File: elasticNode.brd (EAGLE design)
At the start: 58.2 x 52.5 mm, 135 parts, among them J1 FEMALE_HEADER_2X1, J2 JUMPER, J3 JUMPER, J5 FEMALE_HEADER_10X2, J6 USB_CONNMICRO_SMT, J7 USB_CONNMICRO_SMT, M1 SISS23DN, M2 SISS23DN, M3 SISS23DN, M4 SISS23DN, U1 AT90USB128, U10 LTC3419DFN, U11 PAC1720, U14 LTC3419DFN, U2 IS66WV51216EALL, U3 MRF24J40MA, U4 SPARTAN7-LX15, U5 ATMEGA32U4QFN, U6 SST26VF032BWDFN, U7 PAC1720, U8 PAC1720, U9 PAC1720, X1 8MHz, X2 50MHz, X3 32MHz, X4 100MHz, X5 8MHz

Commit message: backup
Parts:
- R29: value 15k -> 0
- moved R1 163.6 mm to (47.4, 21.0)
- moved R2 163.6 mm to (47.4, 19.3)
- moved R54 119.1 mm to (50.6, 41.8), turned to 0 degrees
- moved D9 100.9 mm to (47.4, 17.4), turned to 180 degrees
- moved R29 100.2 mm to (50.6, 40.3)
- moved R33 98.1 mm to (47.4, 15.7), turned to 180 degrees
- moved R26 90.5 mm to (7.20, 49.4), flipped to the bottom, turned to 180 degrees
- moved U7 87.6 mm to (10.9, 50.3), flipped to the bottom
- moved C12 87.1 mm to (28.4, 39.9), turned to 90 degrees
- moved R23 81.2 mm to (14.7, 51.2), flipped to the bottom, turned to 0 degrees
- moved R20 80.8 mm to (14.7, 49.4), flipped to the bottom, turned to 0 degrees
- moved R28 77.1 mm to (17.6, 49.5), flipped to the bottom, turned to 180 degrees
- moved C32 76.4 mm to (12.1, 31.6), flipped to the bottom
- moved R30 75.8 mm to (36.9, 36.7), turned to 0 degrees
- moved U9 73.8 mm to (21.4, 50.3), flipped to the bottom
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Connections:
- net DAUGHTER_VCC: now also R24.1, U8.2; no longer R43.1, U11.2
- net WIRELESS_VCC: now also R43.1, U11.2; no longer R24.1, U8.2
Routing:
- removed copper zone on layer 16, net 1V
- removed copper zone on layer 16, net 3V3
- removed copper zone on layer 16, net 5V
- removed copper zone on layer 16, net N$1
- removed copper zone on layer 16, net N$8
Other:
- board text added: "FPGA LEDS"
- board text added: "MON LEDS"
- board text removed: "FPGA"
- board text removed: "LEDS"

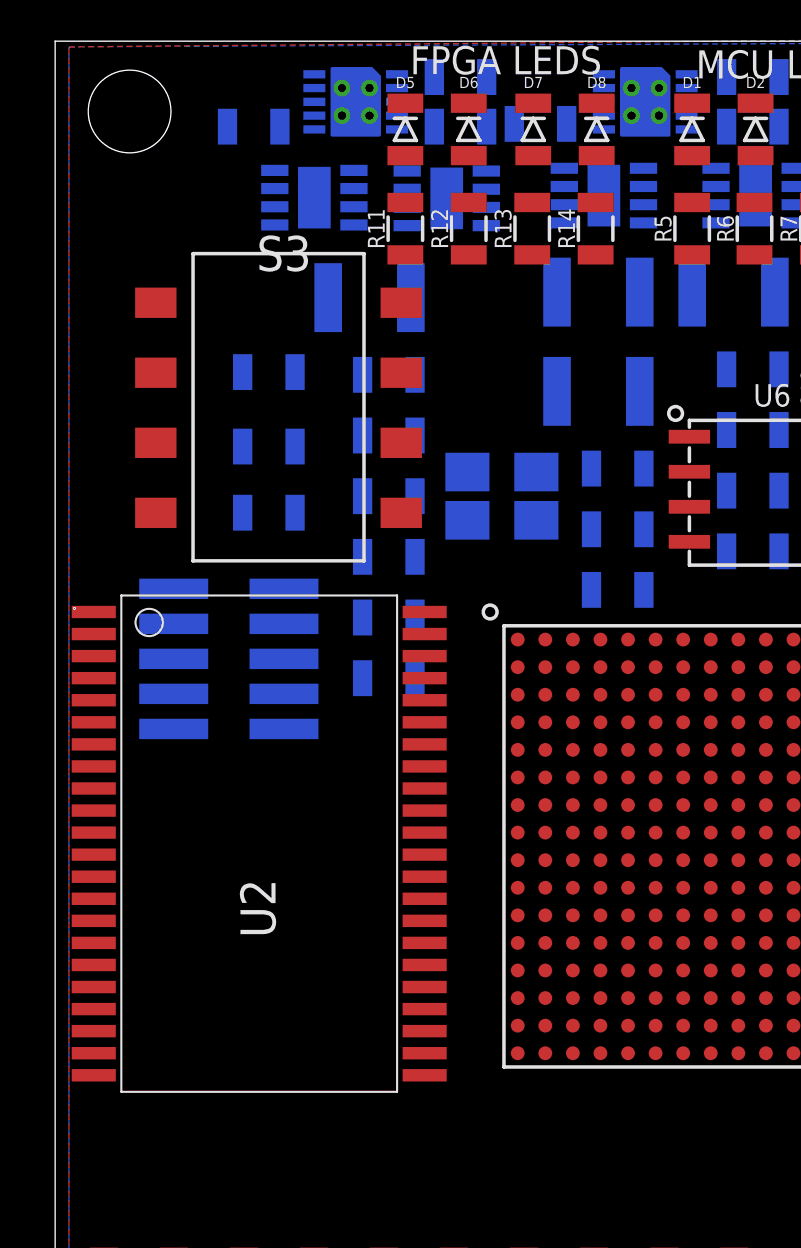
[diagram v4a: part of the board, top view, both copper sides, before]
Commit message: backup
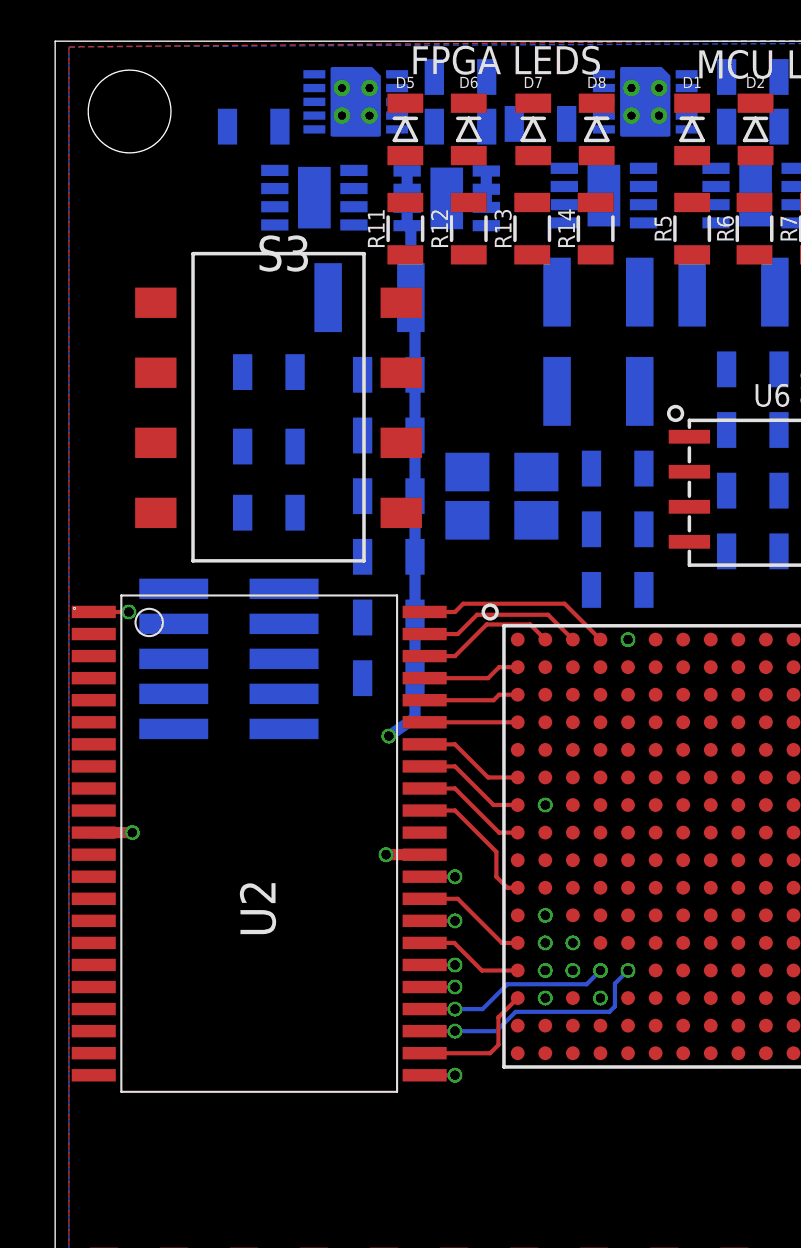
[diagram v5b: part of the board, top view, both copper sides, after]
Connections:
- net SRAM_A0: no longer U4.D3
- net SRAM_A1: no longer U4.C3
- net SRAM_A10: now also U4.M5; no longer U4.C5
- net SRAM_A11: now also U4.N1; no longer U4.C4
- net SRAM_A12: no longer U4.E4
- net SRAM_A13: no longer U4.D4
- net SRAM_A14: no longer U4.F3
- net SRAM_A15: no longer U4.F2
- net SRAM_A16: no longer U4.G1
- net SRAM_A17: now also U4.N4; no longer U4.F1
- net SRAM_A18: now also U4.M2; no longer U4.E2
- net SRAM_A2: no longer U4.A4
- net SRAM_A3: no longer U4.A3
- net SRAM_A4: now also U4.A5; no longer U4.B3
- net SRAM_A5: now also U4.A4; no longer U4.A2
- net SRAM_A6: now also U4.A3; no longer U4.B5
- net SRAM_A7: now also U4.A2; no longer U4.A5
- net SRAM_A8: now also U4.M3; no longer U4.B2
- net SRAM_A9: now also U4.M4; no longer U4.B1
- net SRAM_CS: no longer U4.B6
- net SRAM_D0: no longer U4.D2
- net SRAM_D1: no longer U4.D1
- net SRAM_D10: now also U4.L1; no longer U4.K3
- net SRAM_D11: now also U4.L2; no longer U4.J4
- net SRAM_D12: now also U4.J1; no longer U4.J3
- net SRAM_D13: now also U4.H1; no longer U4.M1
- net SRAM_D14: now also U4.G1; no longer U4.L1
- net SRAM_D15: now also U4.F1; no longer U4.M3
- net SRAM_D2: no longer U4.C1
- net SRAM_D3: no longer U4.H4
- net SRAM_D4: no longer U4.H3
- net SRAM_D5: no longer U4.H2
- net SRAM_D6: no longer U4.H1
- net SRAM_D7: no longer U4.J2
- net SRAM_D8: now also U4.M1; no longer U4.J1
- net SRAM_D9: now also U4.L3; no longer U4.K4
- net SRAM_LB: now also U4.D1; no longer U4.N1
- net SRAM_OE: now also U4.B1; no longer U4.M2
- net SRAM_UB: now also U4.C1; no longer U4.P2
- net SRAM_WE: no longer U4.F4
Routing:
- net SRAM_VDD: track 0.00 -> 56.4 mm, vias 0 -> 6
- net SRAM_A4: track 0.00 -> 19.8 mm, vias 0 -> 2
- net SRAM_A10: track 0.00 -> 8.77 mm, vias 0 -> 2
- net SRAM_A17: track 0.00 -> 8.73 mm, vias 0 -> 2
- net SRAM_A5: track 0.00 -> 7.04 mm
- net SRAM_A9: track 0.00 -> 6.95 mm, vias 0 -> 2
- net SRAM_D9: track 0.00 -> 6.24 mm, vias 0 -> 2
- net SRAM_A6: track 0.00 -> 6.04 mm
- net SRAM_A8: track 0.00 -> 5.62 mm, vias 0 -> 2
- net SRAM_A7: track 0.00 -> 5.08 mm
- net SRAM_D12: track 0.00 -> 5.06 mm
- net SRAM_A11: track 0.00 -> 4.79 mm
- net SRAM_D11: track 0.00 -> 4.77 mm, vias 0 -> 2
- net SRAM_A18: track 0.00 -> 4.46 mm, vias 0 -> 2
- net SRAM_D10: track 0.00 -> 4.04 mm
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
